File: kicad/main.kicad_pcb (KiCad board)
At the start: 2 copper layers, 135.9 x 160 mm, 46 parts, among them J1 Barrel_Jack, J2 UART, P1 Mini-DIN_6pins_ver3, SW1 Reset, SW2 SW_Push_DPDT, U1 KM1810VM88, U10 L7805, U11 15 MHz, U12 8255, U13 uSD adapter, U14 8259, U15 AS6C4008-55PCN, U16 16550, U18 1.8432 MHz, U2 W27C512, U3 AS6C4008-55PCN, U4 74HC573, U5 74HC573, U6 GAL22V10, U7 DS1813-5+, U8 74HC14, U9 8253

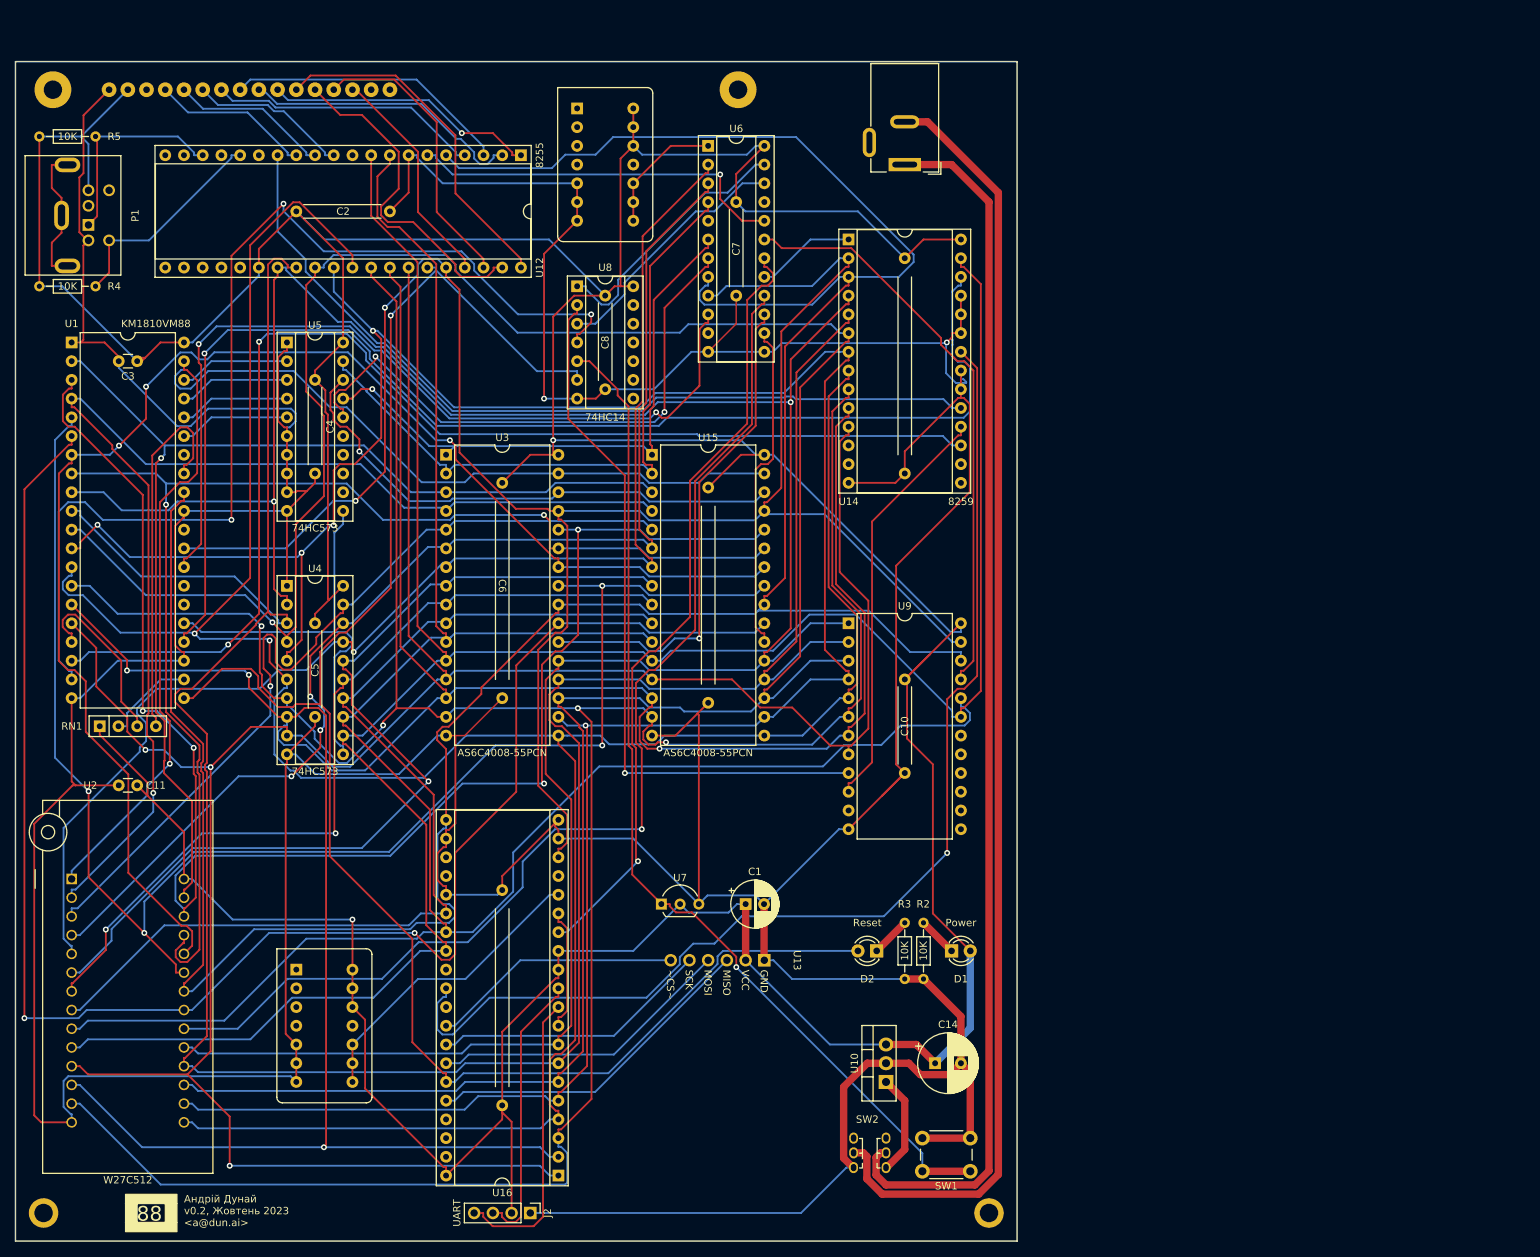
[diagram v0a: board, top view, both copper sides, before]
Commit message: PCB 2.0 RC
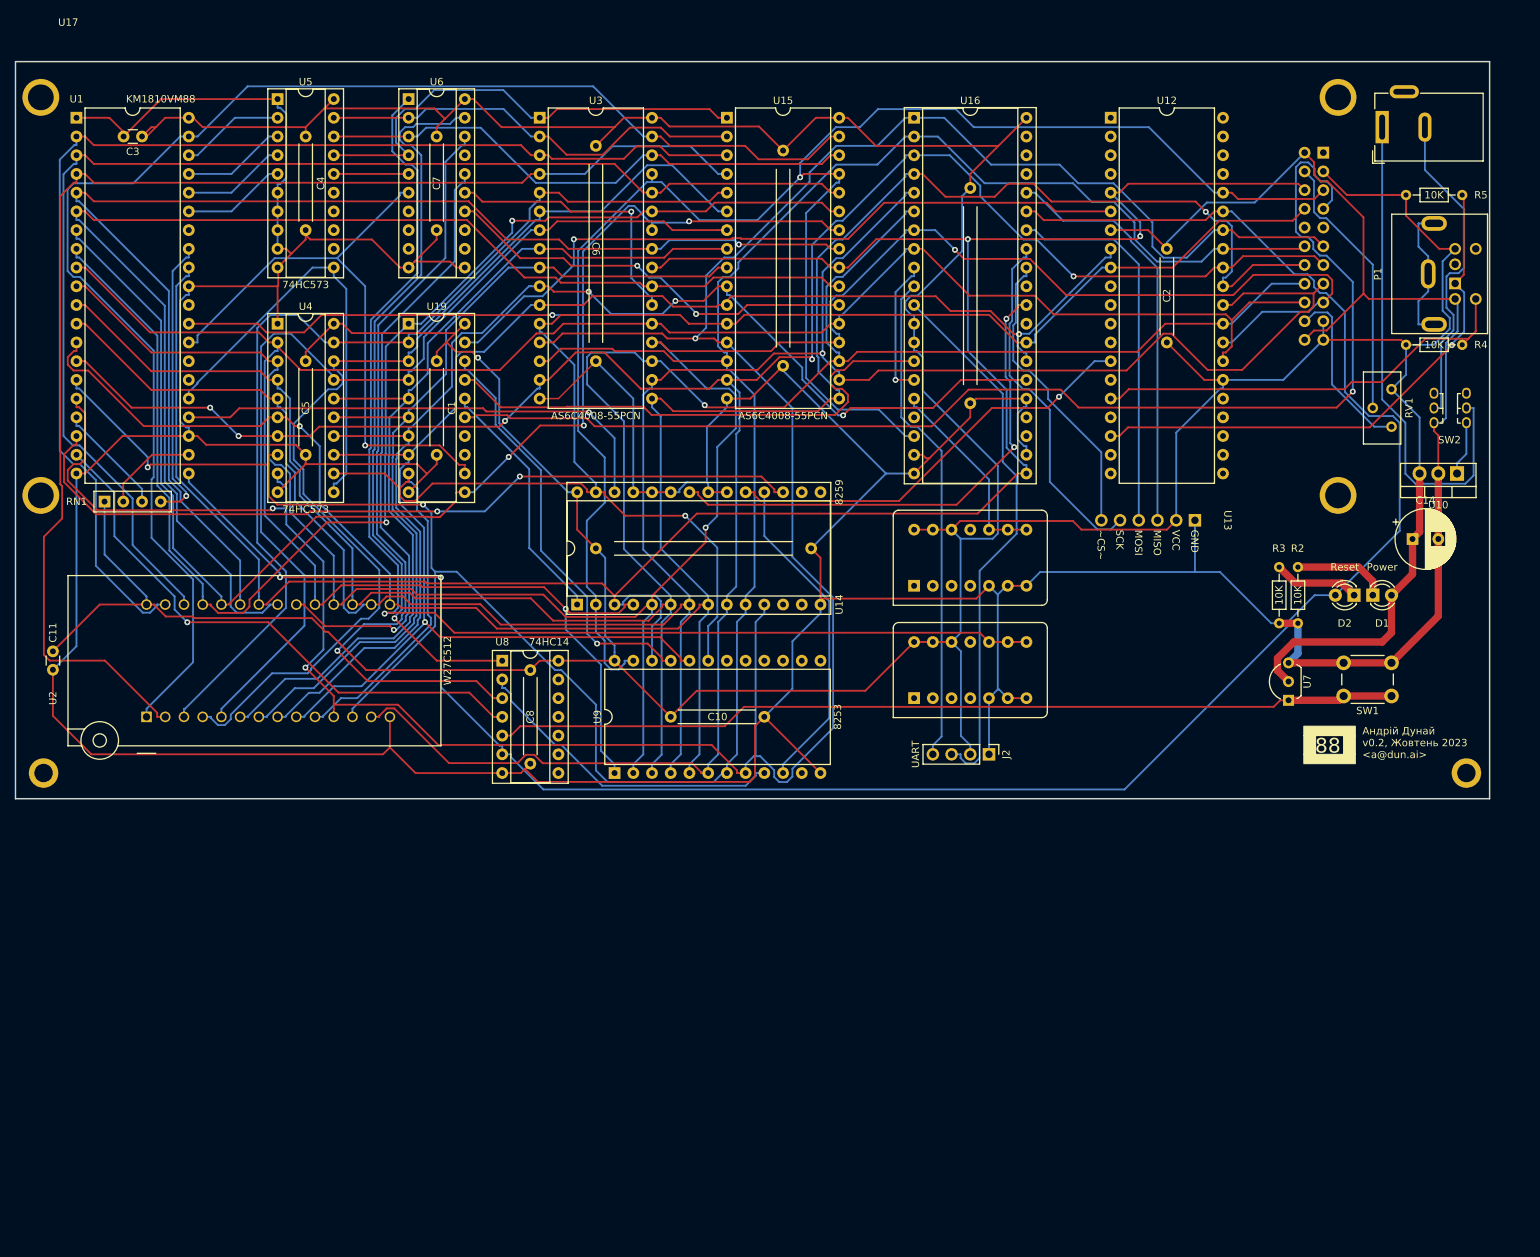
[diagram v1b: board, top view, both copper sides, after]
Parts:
- removed LCD1: ~, footprints:2004A-OLED
- added RV1: R_Potentiometer, Potentiometer_THT:Potentiometer_Bourns_3296Y_Vertical, F.Cu at (207.0, 67.3)
- added U17: T6963C, footprints:LCD24064, F.Cu at (21.8, 17.1)
- added U19: ATF16V8, Package_DIP:DIP-20_W7.62mm_Socket, F.Cu at (73.7, 53.3)
- C1: value 10 uF -> 0.1 uF; footprint Capacitor_THT:CP_Radial_D6.3mm_P2.50mm -> footprints:C_Disc_Long
- U12: footprint Package_DIP:DIP-40_W15.24mm_Socket -> Package_DIP:DIP-40_W15.24mm
- U6: value GAL22V10 -> ATF16V8; footprint Package_DIP:DIP-24_W7.62mm_Socket -> Package_DIP:DIP-20_W7.62mm_Socket
- moved P1 185.6 mm to (215.6, 47.9)
- moved R4 185.6 mm to (209.0, 56.2)
- moved R5 185.6 mm to (209.0, 35.9)
- moved U16 151.4 mm to (142.2, 25.4), turned to 0 degrees
- moved C9 128.5 mm to (149.9, 41.3), turned to -90 degrees
- moved SW2 128.1 mm to (212.1, 61.9)
- moved C2 119.4 mm to (176.5, 55.9), turned to 90 degrees
- moved U10 113.2 mm to (215.9, 73.7), turned to 180 degrees
- moved U18 108.3 mm to (149.9, 85.3), turned to 0 degrees
- moved C14 96.2 mm to (209.9, 82.5)
- moved U7 89.5 mm to (193.0, 104.4), turned to 90 degrees
- moved H2 88.1 mm to (217.2, 114.3)
- moved J2 88.0 mm to (152.4, 111.8)
- moved SW1 86.2 mm to (207.0, 103.8)
- moved U11 84.8 mm to (149.9, 100.5), turned to 0 degrees
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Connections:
- U12 pad 1: Net-(LCD1-D_{3}) -> unconnected-(U12-PA3-Pad1)
- U12 pad 11: Net-(LCD1-E) -> unconnected-(U12-PC6-Pad11)
- U12 pad 12: Net-(LCD1-R~{W}) -> unconnected-(U12-PC5-Pad12)
- U12 pad 13: Net-(LCD1-RS) -> unconnected-(U12-PC4-Pad13)
- U12 pad 2: Net-(LCD1-D_{2}) -> unconnected-(U12-PA2-Pad2)
- U12 pad 3: Net-(LCD1-D_{1}) -> unconnected-(U12-PA1-Pad3)
- U12 pad 37: Net-(LCD1-D_{7}) -> unconnected-(U12-PA7-Pad37)
- U12 pad 38: Net-(LCD1-D_{6}) -> unconnected-(U12-PA6-Pad38)
- U12 pad 39: Net-(LCD1-D_{5}) -> unconnected-(U12-PA5-Pad39)
- U12 pad 4: Net-(LCD1-D_{0}) -> unconnected-(U12-PA0-Pad4)
- U12 pad 40: Net-(LCD1-D_{4}) -> unconnected-(U12-PA4-Pad40)
- U14 pad 1: INT~{EN} -> PIC~{EN}
- U6 pad 10: IO/~{M} -> GND
- U6 pad 11: unconnected-(U6-I-Pad11) -> GND
- U6 pad 12: GND -> unconnected-(U6-I/O-Pad12)
- U6 pad 13: GND -> unconnected-(U6-I/O-Pad13)
- U6 pad 17: INT~{EN} -> unconnected-(U6-I/O-Pad17)
- U6 pad 18: UART~{EN} -> Net-(U6-I/O-Pad18)
- U6 pad 19: TIMER~{EN} -> Net-(U6-I/O-Pad19)
- U6 pad 2: A_{5} -> A_{16}
- U6 pad 20: PPI~{EN} -> +5V
- U6 pad 3: A_{6} -> A_{17}
- U6 pad 4: A_{16} -> A_{18}
- U6 pad 5: A_{17} -> A_{19}
- U6 pad 6: A_{18} -> IO/~{M}
- U6 pad 7: A_{19} -> unconnected-(U6-I-Pad7)
- U6 pad 8: ~{RD} -> unconnected-(U6-I-Pad8)
- U6 pad 9: ~{WR} -> unconnected-(U6-I-Pad9)
- U8 pad 1: Net-(U6-I/O/Q-Pad23) -> Net-(U6-I/O-Pad19)
- U8 pad 3: Net-(U6-I/O/Q-Pad22) -> Net-(U6-I/O-Pad18)
- U9 pad 21: TIMER~{EN} -> PIT~{EN}
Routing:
- net LCD~{EN}: track 0.00 -> 170.4 mm, vias 0 -> 1
- net MCLK: track 17.3 -> 167.1 mm, vias 0 -> 1
- net Net-(J1-Pad2): track 174.7 -> 44.1 mm
- net Net-(U6-I/O-Pad18): track 0.00 -> 108.0 mm, vias 0 -> 1
- net ~{INTA}: track 173.1 -> 67.3 mm
- net GND: track 881.9 -> 777.3 mm, vias 2 -> 0
- net Net-(U6-I/O-Pad19): track 0.00 -> 99.0 mm, vias 0 -> 1
- net Net-(J1-Pad1): track 165.6 -> 68.7 mm
- net INT4: track 157.7 -> 69.8 mm, vias 1 -> 2
- net A_{1}: track 301.1 -> 218.1 mm, vias 0 -> 2
- net TIMER~{EN}: track 79.1 -> 0.00 mm
- net ROM~{EN}: track 156.0 -> 84.2 mm
- net CLK: track 148.4 -> 77.0 mm, vias 3 -> 1
- net A_{19}: track 78.8 -> 10.2 mm, vias 2 -> 0
- net A_{0}: track 327.4 -> 261.9 mm, vias 0 -> 1
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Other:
- board size 135.9 x 160 mm -> 200 x 100 mm
